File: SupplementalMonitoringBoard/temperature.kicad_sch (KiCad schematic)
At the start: 10 parts, among them U3 INA180B1

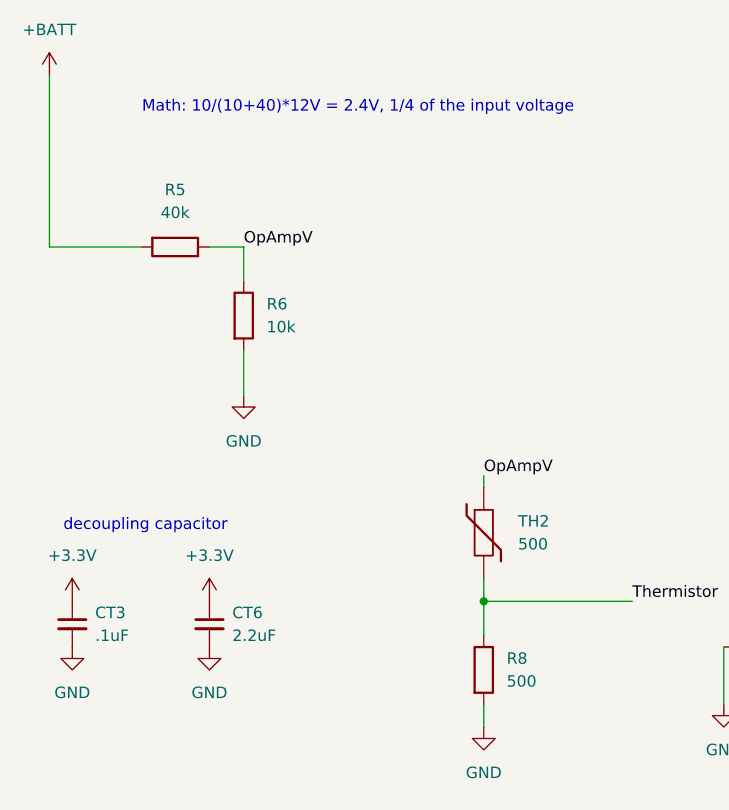
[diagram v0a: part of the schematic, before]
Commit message: Supplemental MOnitoring Board
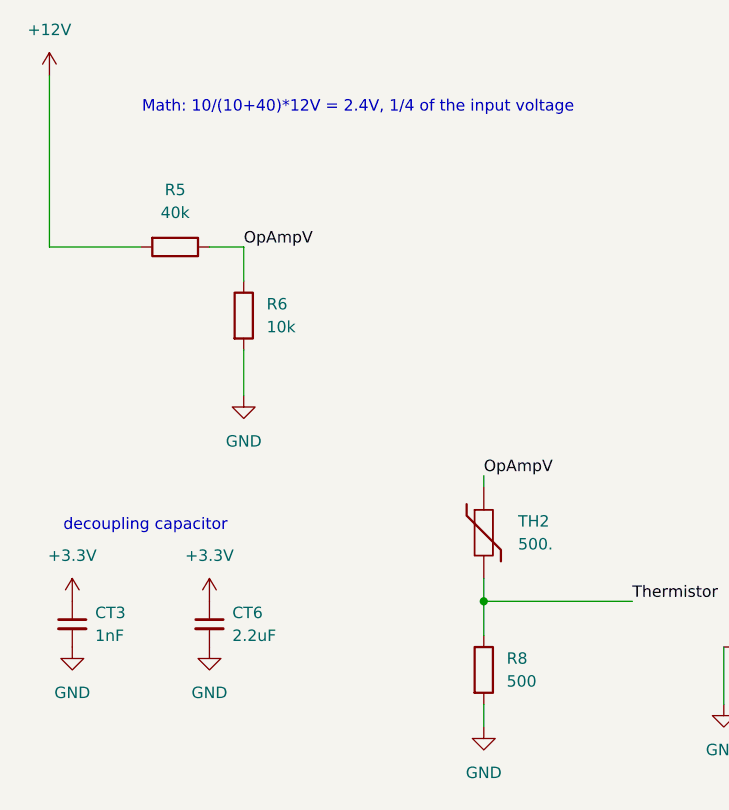
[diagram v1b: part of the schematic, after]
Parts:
- CT3: value .1uF -> 1nF; P/N (none) -> C0805C102J5HACAUTO
- CT6: P/N (none) -> UMK212ABJ225KG-T
- R12, R13, R6: P/N (none) -> CRCW080510K0FKEAC
- R15: P/N (none) -> 0805W8F3001T5E
- R5: P/N (none) -> CRCW080540K0FKEA
- R8: P/N (none) -> RN73R2ATTD5000B25
- TH2: value 500 -> 500.; P/N (none) -> TFPT0805L5001FM
- U3: P/N (none) -> SBOS741H
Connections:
- net +BATT renamed +12V
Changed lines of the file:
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@@
 			)
 		)
-		(property "Datasheet" "~"
+		(property "Datasheet" "https://www.mouser.com/ProductDetail/Murata-Electronics/GRM219R6YA475KA73D?qs=eeBpzGFlv%252B%252Bho6epIC%2FPCA%3D%3D"
 			(at 49.53 91.44 0)
 			(effects
@@
 			)
 		)
+		(property "P/N" "UMK212ABJ225KG-T"
+			(at 49.53 91.44 0)
+			(effects
+				(font
+					(size 1.27 1.27)
+				)
+				(hide yes)
+			)
+		)
 		(pin "1"
 		)
@@
 			)
 		)
-		(property "Datasheet" "~"
+		(property "Datasheet" "https://www.mouser.com/datasheet/2/447/PYu_RT_1_to_0_01_RoHS_L_15-3461507.pdf"
 			(at 53.34 57.15 0)
 			(effects
@@
 		)
 		(property "Description" "Resistor"
+			(at 53.34 57.15 0)
+			(effects
+				(font
+					(size 1.27 1.27)
+				)
+				(hide yes)
+			)
+		)
+		(property "P/N" "CRCW080510K0FKEAC"
 			(at 53.34 57.15 0)
 			(effects
@@
 			)
 		)
-		(property "Value" "500"
+		(property "Value" "500."
 			(at 83.82 82.5499 0)
 			(effects
@@
 			)
 		)
-		(property "Datasheet" "~"
+		(property "Datasheet" "https://www.vishay.com/docs/33017/tfpt.pdf"
 			(at 80.01 81.28 0)
 			(effects
@@
 		)
 		(property "Description" "Temperature dependent resistor"
+			(at 80.01 81.28 0)
+			(effects
+				(font
+					(size 1.27 1.27)
+				)
+				(hide yes)
+			)
+		)
+		(property "P/N" "TFPT0805L5001FM"
 			(at 80.01 81.28 0)
 			(effects
@@
 			)
 		)
-		(property "Datasheet" "~"
+		(property "Datasheet" "https://www.koaspeer.com/pdfs/RN73R.pdf"
 			(at 80.01 96.52 0)
 			(effects
@@
 		)
 		(property "Description" "Resistor"
+			(at 80.01 96.52 0)
+			(effects
+				(font
+					(size 1.27 1.27)
+				)
+				(hide yes)
+			)
+		)
+		(property "P/N" "RN73R2ATTD5000B25"
 			(at 80.01 96.52 0)
 			(effects
@@
 			)
 		)
-		(property "Value" ".1uF"
+		(property "Value" "1nF"
 			(at 36.83 92.7162 0)
 			(effects
@@
 			)
 		)
-		(property "Datasheet" "~"
+		(property "Datasheet" "https://www.mouser.com/ProductDetail/KEMET/C0805C102J5HACAUTO?qs=j%252B1pi9TdxUbgwPgoM1tuTw%3D%3D"
 			(at 34.29 91.44 0)
 			(effects
@@
 		)
 		(property "Description" "Unpolarized capacitor, small symbol"
+			(at 34.29 91.44 0)
+			(effects
+				(font
+					(size 1.27 1.27)
+				)
+				(hide yes)
+			)
+		)
+		(property "P/N" "C0805C102J5HACAUTO"
 			(at 34.29 91.44 0)
 			(effects
@@
 			)
 		)
-		(property "Datasheet" "~"
+		(property "Datasheet" "https://www.mouser.com/datasheet/2/447/PYu_RT_1_to_0_01_RoHS_L_15-3461507.pdf"
 			(at 133.35 100.33 0)
 			(effects
@@
 		)
 		(property "Description" "Resistor"
+			(at 133.35 100.33 0)
+			(effects
+				(font
+					(size 1.27 1.27)
+				)
+				(hide yes)
+			)
+		)
+		(property "P/N" "CRCW080510K0FKEAC"
 			(at 133.35 100.33 0)
 			(effects
@@
 			)
 		)
+		(property "P/N" "SBOS741H "
+			(at 152.4 91.44 0)
+			(effects
+				(font
+					(size 1.27 1.27)
+				)
+				(hide yes)
+			)
+		)
 		(pin "1"
 		)
@@
 			)
 		)
-		(property "Datasheet" "~"
+		(property "Datasheet" "https://www.vishay.com/docs/20035/dcrcwe3.pdf"
 			(at 45.72 49.53 0)
 			(effects
@@
 		)
 		(property "Description" "Resistor"
+			(at 45.72 49.53 0)
+			(effects
+				(font
+					(size 1.27 1.27)
+				)
+				(hide yes)
+			)
+		)
+		(property "P/N" "CRCW080540K0FKEA"
 			(at 45.72 49.53 0)
 			(effects
@@
 			)
 		)
-		(property "Datasheet" "~"
+		(property "Datasheet" "https://www.mouser.com/datasheet/2/1365/1-3044649.pdf"
 			(at 156.21 106.68 0)
 			(effects
@@
 			)
 		)
+		(property "P/N" "0805W8F3001T5E"
+			(at 156.21 106.68 0)
+			(effects
+				(font
+					(size 1.27 1.27)
+				)
+				(hide yes)
+			)
+		)
 		(pin "1"
 		)
@@
 	)
 	(symbol
-		(lib_id "power:+BATT")
+		(lib_id "power:+3.3V")
+		(at 34.29 88.9 0)
+		(unit 1)
+		(exclude_from_sim no)
+		(in_bom yes)
+		(on_board yes)
+		(dnp no)
+		(property "Reference" "#PWR021"
+			(at 34.29 92.71 0)
+			(effects
+				(font
+					(size 1.27 1.27)
+				)
+				(hide yes)
+			)
+		)
+		(property "Value" "+3.3V"
+			(at 34.29 83.82 0)
+			(effects
+				(font
+					(size 1.27 1.27)
+				)
+			)
+		)
+		(property "Footprint" ""
+			(at 34.29 88.9 0)
+			(effects
+				(font
+					(size 1.27 1.27)
+				)
+				(hide yes)
+			)
+		)
+		(property "Datasheet" ""
+			(at 34.29 88.9 0)
+			(effects
+				(font
+					(size 1.27 1.27)
+				)
+				(hide yes)
+			)
+		)
+		(property "Description" "Power symbol creates a global label with name \"+3.3V\""
+			(at 34.29 88.9 0)
+			(effects
+				(font
+					(size 1.27 1.27)
+				)
+				(hide yes)
+			)
+		)
+		(pin "1"
+		)
+		(instances
+			(project "SupplementalMonitoringBoard"
+				(path "/aa0415d0-3287-4bc4-9a8e-766ada9ace2f/cde5a840-cd97-4154-b488-bad27326129c"
+					(reference "#PWR021")
+					(unit 1)
+				)
+			)
+		)
+	)
+	(symbol
+		(lib_id "power:+12V")
 		(at 31.75 30.48 0)
 		(unit 1)
@@
 			)
 		)
-		(property "Value" "+BATT"
+		(property "Value" "+12V"
 			(at 31.75 25.4 0)
 			(effects
@@
 			)
 		)
-		(property "Description" "Power symbol creates a global label with name \"+BATT\""
+		(property "Description" "Power symbol creates a global label with name \"+12V\""
 			(at 31.75 30.48 0)
 			(effects
@@
 				(path "/aa0415d0-3287-4bc4-9a8e-766ada9ace2f/cde5a840-cd97-4154-b488-bad27326129c"
 					(reference "#PWR025")
-					(unit 1)
-				)
-			)
-		)
-	)
-	(symbol
-		(lib_id "power:+3.3V")
-		(at 34.29 88.9 0)
-		(unit 1)
-		(exclude_from_sim no)
-		(in_bom yes)
-		(on_board yes)
-		(dnp no)
-		(property "Reference" "#PWR021"
-			(at 34.29 92.71 0)
-			(effects
-				(font
-					(size 1.27 1.27)
-				)
-				(hide yes)
-			)
-		)
-		(property "Value" "+3.3V"
-			(at 34.29 83.82 0)
-			(effects
-				(font
-					(size 1.27 1.27)
-				)
-			)
-		)
-		(property "Footprint" ""
-			(at 34.29 88.9 0)
-			(effects
-				(font
-					(size 1.27 1.27)
-				)
-				(hide yes)
-			)
-		)
-		(property "Datasheet" ""
-			(at 34.29 88.9 0)
-			(effects
-				(font
-					(size 1.27 1.27)
-				)
-				(hide yes)
-			)
-		)
-		(property "Description" "Power symbol creates a global label with name \"+3.3V\""
-			(at 34.29 88.9 0)
-			(effects
-				(font
-					(size 1.27 1.27)
-				)
-				(hide yes)
-			)
-		)
-		(pin "1"
-		)
-		(instances
-			(project "SupplementalMonitoringBoard"
-				(path "/aa0415d0-3287-4bc4-9a8e-766ada9ace2f/cde5a840-cd97-4154-b488-bad27326129c"
-					(reference "#PWR021")
 					(unit 1)
 				)
@@
 			)
 		)
-		(property "Datasheet" "~"
+		(property "Datasheet" "https://www.mouser.com/datasheet/2/447/PYu_RT_1_to_0_01_RoHS_L_15-3461507.pdf"
 			(at 110.49 93.98 0)
 			(effects
@@
 			(at 110.49 93.98 0)
 			(effects
+				(font
+					(size 1.27 1.27)
+				)
+				(hide yes)
+			)
+		)
+		(property "P/N" "CRCW080510K0FKEAC"
+			(at 110.49 93.98 0)
+			(effects
